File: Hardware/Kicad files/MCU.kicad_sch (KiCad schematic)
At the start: 1 part, among them U201 NUCLEO-H753ZI

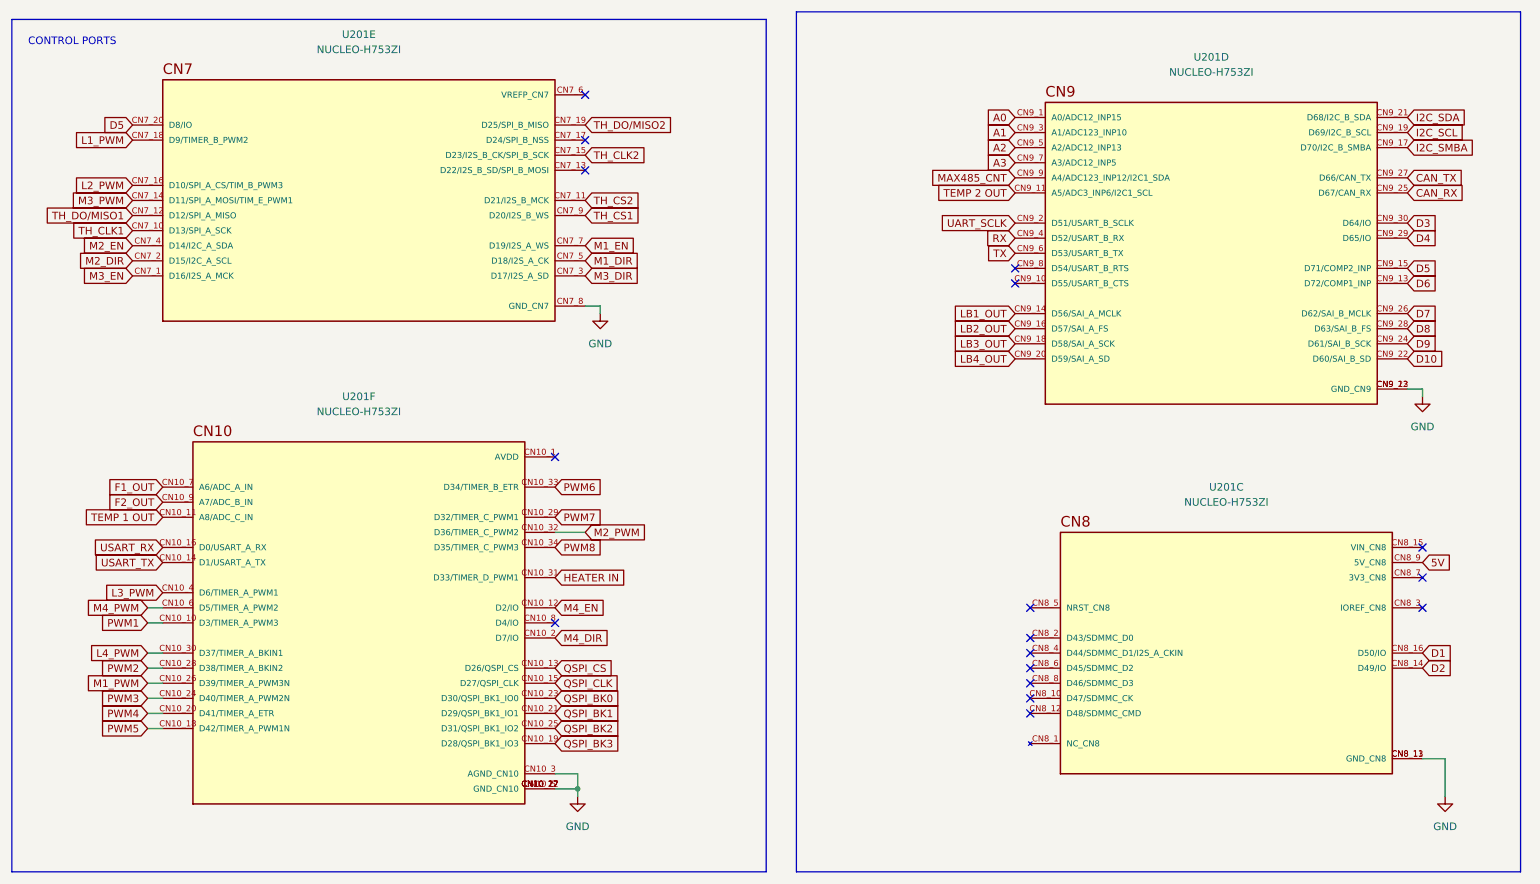
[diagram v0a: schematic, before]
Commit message: Add files via upload
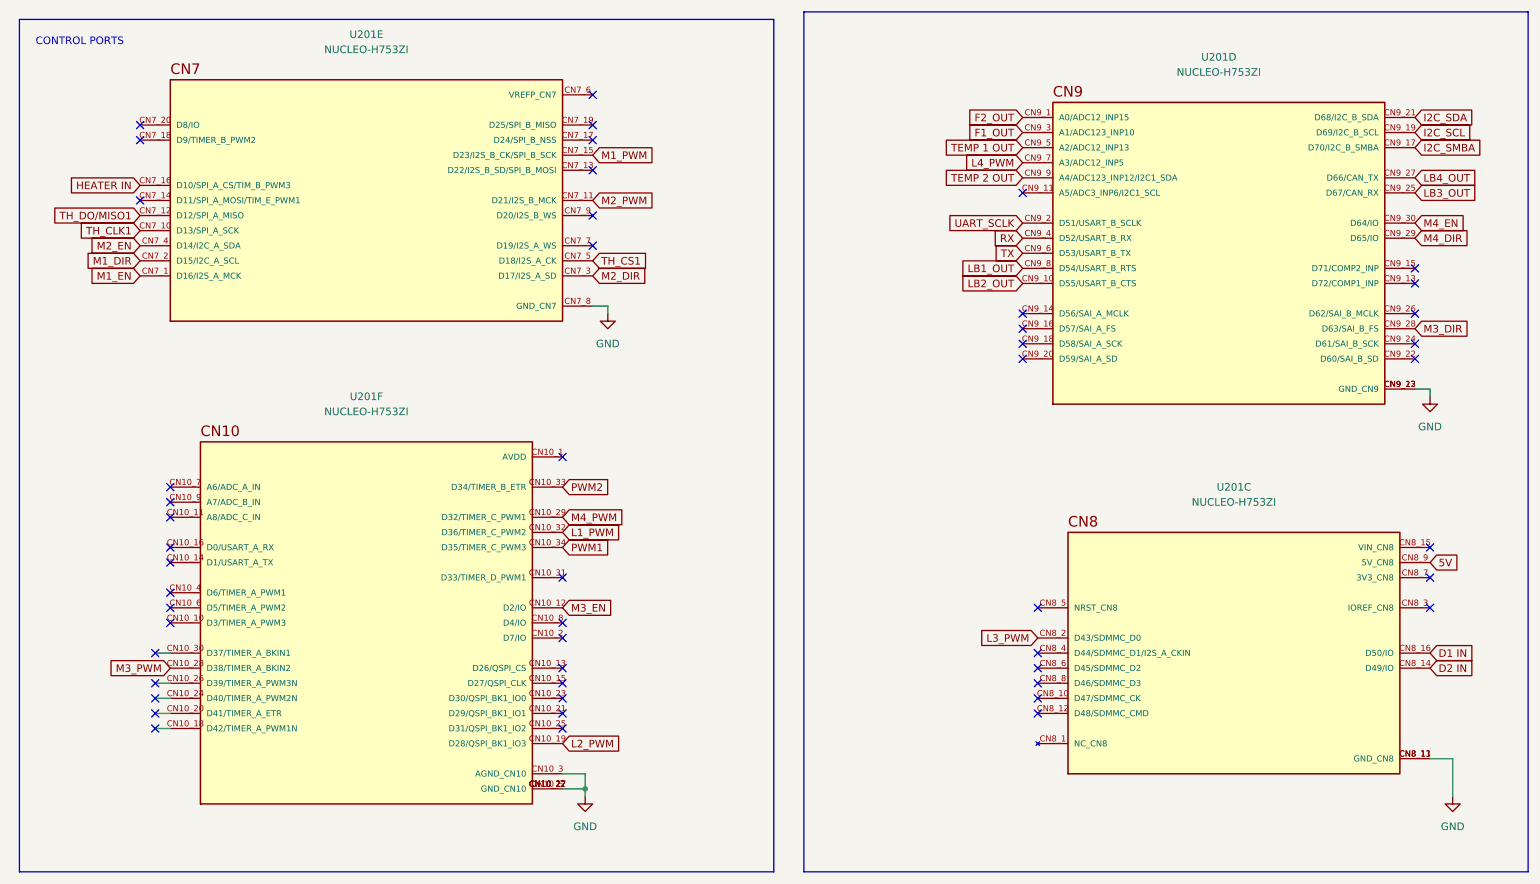
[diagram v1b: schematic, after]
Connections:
- net A0 is gone; now on net F2_OUT: U201.CN9_1 (A0/ADC12_INP15)
- net A1 is gone; now on net F1_OUT: U201.CN9_3 (A1/ADC123_INP10)
- net A2 is gone; now on net TEMP 1 OUT: U201.CN9_5 (A2/ADC12_INP13)
- net A3 is gone; now on net L4_PWM: U201.CN9_7 (A3/ADC12_INP5)
- net CAN_RX is gone; now on net LB3_OUT: U201.CN9_25 (D67/CAN_RX)
- net CAN_TX is gone; now on net LB4_OUT: U201.CN9_27 (D66/CAN_TX)
- net D3 is gone; now on net M4_EN: U201.CN9_30 (D64/IO)
- net D4 is gone; now on net M4_DIR: U201.CN9_29 (D65/IO)
- net D8 is gone; now on net M3_DIR: U201.CN9_28 (D63/SAI_B_FS)
- net MAX485_CNT is gone; now on net TEMP 2 OUT: U201.CN9_9 (A4/ADC123_INP12/I2C1_SDA)
- net PWM6 is gone; now on net PWM2: U201.CN10_33 (D34/TIMER_B_ETR)
- net PWM7 is gone; now on net M4_PWM: U201.CN10_29 (D32/TIMER_C_PWM1)
- net PWM8 is gone; now on net PWM1: U201.CN10_34 (D35/TIMER_C_PWM3)
- net QSPI_BK3 is gone; now on net L2_PWM: U201.CN10_19 (D28/QSPI_BK1_IO3)
- net TH_CLK2 is gone; now on net M1_PWM: U201.CN7_15 (D23/I2S_B_CK/SPI_B_SCK)
- net TH_CS2 is gone; now on net M2_PWM: U201.CN7_11 (D21/I2S_B_MCK)
- net F1_OUT: no longer U201.CN10_7 (A6/ADC_A_IN)
- net F2_OUT: no longer U201.CN10_9 (A7/ADC_B_IN)
- net HEATER IN: now also U201.CN7_16 (D10/SPI_A_CS/TIM_B_PWM3); no longer U201.CN10_31 (D33/TIMER_D_PWM1)
- net L1_PWM: now also U201.CN10_32 (D36/TIMER_C_PWM2); no longer U201.CN7_18 (D9/TIMER_B_PWM2)
- net L2_PWM: no longer U201.CN7_16 (D10/SPI_A_CS/TIM_B_PWM3)
- net L3_PWM: now also U201.CN8_2 (D43/SDMMC_D0); no longer U201.CN10_4 (D6/TIMER_A_PWM1)
- net L4_PWM: no longer U201.CN10_30 (D37/TIMER_A_BKIN1)
- net LB1_OUT: now also U201.CN9_8 (D54/USART_B_RTS); no longer U201.CN9_14 (D56/SAI_A_MCLK)
- net LB2_OUT: now also U201.CN9_10 (D55/USART_B_CTS); no longer U201.CN9_16 (D57/SAI_A_FS)
- net LB3_OUT: no longer U201.CN9_18 (D58/SAI_A_SCK)
- net LB4_OUT: no longer U201.CN9_20 (D59/SAI_A_SD)
- net M1_DIR: now also U201.CN7_2 (D15/I2C_A_SCL); no longer U201.CN7_5 (D18/I2S_A_CK)
- net M1_EN: now also U201.CN7_1 (D16/I2S_A_MCK); no longer U201.CN7_7 (D19/I2S_A_WS)
- net M1_PWM: no longer U201.CN10_26 (D39/TIMER_A_PWM3N)
- net M2_DIR: now also U201.CN7_3 (D17/I2S_A_SD); no longer U201.CN7_2 (D15/I2C_A_SCL)
- net M2_PWM: no longer U201.CN10_32 (D36/TIMER_C_PWM2)
- net M3_DIR: no longer U201.CN7_3 (D17/I2S_A_SD)
- net M3_EN: now also U201.CN10_12 (D2/IO); no longer U201.CN7_1 (D16/I2S_A_MCK)
- net M3_PWM: now also U201.CN10_28 (D38/TIMER_A_BKIN2); no longer U201.CN7_14 (D11/SPI_A_MOSI/TIM_E_PWM1)
- net M4_DIR: no longer U201.CN10_2 (D7/IO)
- net M4_EN: no longer U201.CN10_12 (D2/IO)
- net M4_PWM: no longer U201.CN10_6 (D5/TIMER_A_PWM2)
- net PWM1: no longer U201.CN10_10 (D3/TIMER_A_PWM3)
- net PWM2: no longer U201.CN10_28 (D38/TIMER_A_BKIN2)
- net TEMP 1 OUT: no longer U201.CN10_11 (A8/ADC_C_IN)
- net TEMP 2 OUT: no longer U201.CN9_11 (A5/ADC3_INP6/I2C1_SCL)
- net TH_CS1: now also U201.CN7_5 (D18/I2S_A_CK); no longer U201.CN7_9 (D20/I2S_B_WS)
- net D1 renamed D1 IN
- net D10: no longer names the net of U201.CN9_22 (D60/SAI_B_SD)
- net D2 renamed D2 IN
- net D5: no longer names the net of U201.CN9_15 (D71/COMP2_INP)
- net D5: no longer U201.CN7_20 (D8/IO)
- net D6: no longer names the net of U201.CN9_13 (D72/COMP1_INP)
- net D7: no longer names the net of U201.CN9_26 (D62/SAI_B_MCLK)
- net D9: no longer names the net of U201.CN9_24 (D61/SAI_B_SCK)
- net PWM3: no longer names the net of U201.CN10_24 (D40/TIMER_A_PWM2N)
- net PWM4: no longer names the net of U201.CN10_20 (D41/TIMER_A_ETR)
- net PWM5: no longer names the net of U201.CN10_18 (D42/TIMER_A_PWM1N)
- net QSPI_BK0: no longer names the net of U201.CN10_23 (D30/QSPI_BK1_IO0)
- net QSPI_BK1: no longer names the net of U201.CN10_21 (D29/QSPI_BK1_IO1)
- net QSPI_BK2: no longer names the net of U201.CN10_25 (D31/QSPI_BK1_IO2)
- net QSPI_CLK: no longer names the net of U201.CN10_15 (D27/QSPI_CLK)
- net QSPI_CS: no longer names the net of U201.CN10_13 (D26/QSPI_CS)
- net TH_DO/MISO2: no longer names the net of U201.CN7_19 (D25/SPI_B_MISO)
- net USART_RX: no longer names the net of U201.CN10_16 (D0/USART_A_RX)
- net USART_TX: no longer names the net of U201.CN10_14 (D1/USART_A_TX)
- no-connect marks 17 -> 50

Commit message: Add files via upload
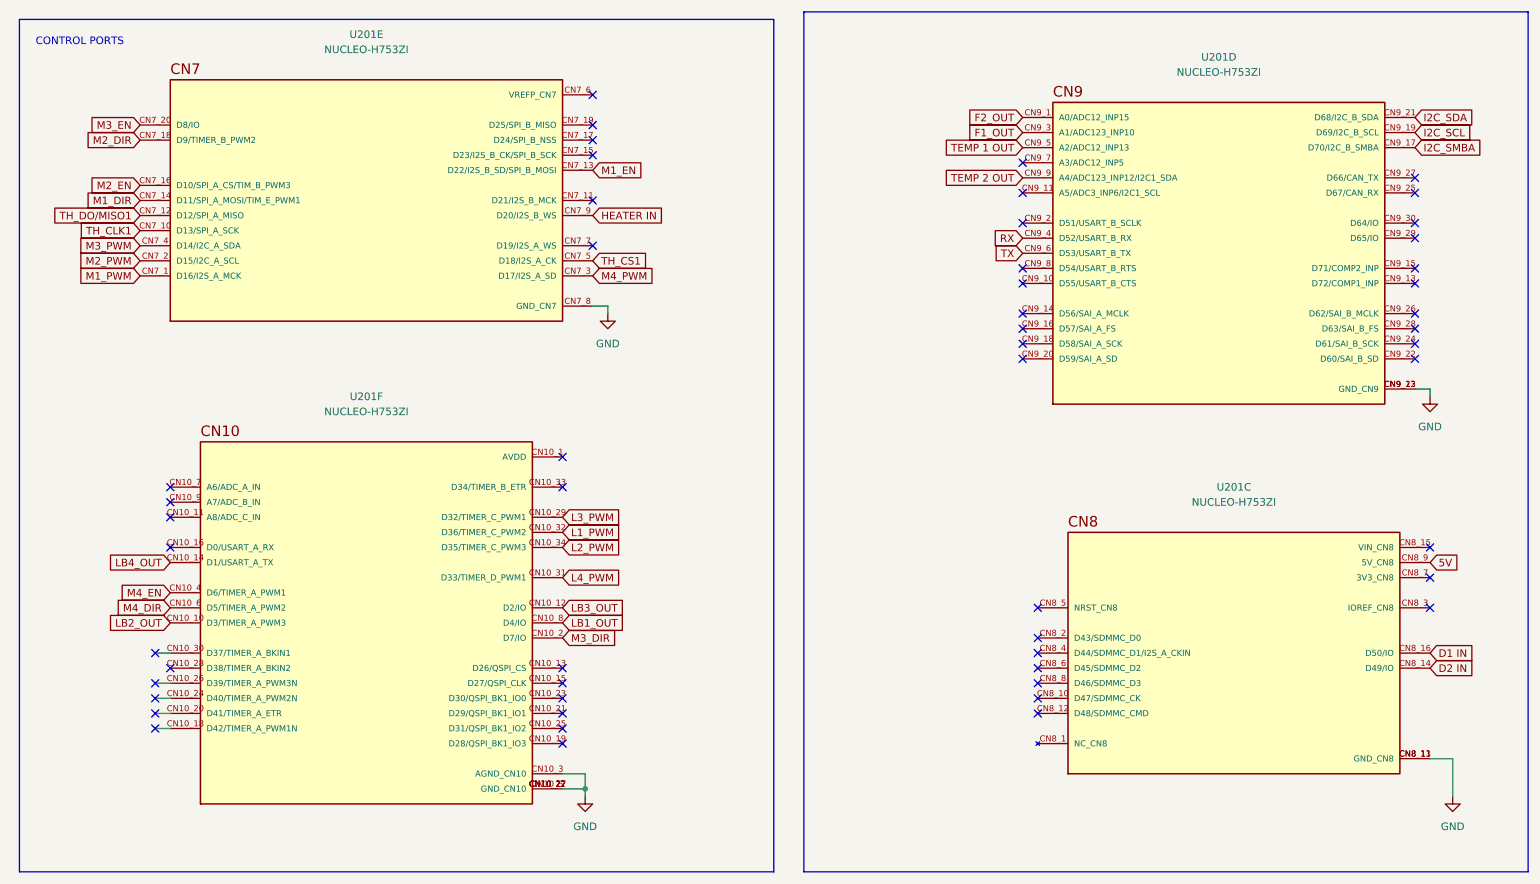
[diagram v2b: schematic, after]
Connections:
- net PWM1 is gone; now on net L2_PWM: U201.CN10_34 (D35/TIMER_C_PWM3)
- net HEATER IN: now also U201.CN7_9 (D20/I2S_B_WS); no longer U201.CN7_16 (D10/SPI_A_CS/TIM_B_PWM3)
- net L2_PWM: no longer U201.CN10_19 (D28/QSPI_BK1_IO3)
- net L3_PWM: now also U201.CN10_29 (D32/TIMER_C_PWM1); no longer U201.CN8_2 (D43/SDMMC_D0)
- net L4_PWM: now also U201.CN10_31 (D33/TIMER_D_PWM1); no longer U201.CN9_7 (A3/ADC12_INP5)
- net LB1_OUT: now also U201.CN10_8 (D4/IO); no longer U201.CN9_8 (D54/USART_B_RTS)
- net LB2_OUT: now also U201.CN10_10 (D3/TIMER_A_PWM3); no longer U201.CN9_10 (D55/USART_B_CTS)
- net LB3_OUT: now also U201.CN10_12 (D2/IO); no longer U201.CN9_25 (D67/CAN_RX)
- net LB4_OUT: now also U201.CN10_14 (D1/USART_A_TX); no longer U201.CN9_27 (D66/CAN_TX)
- net M1_DIR: now also U201.CN7_14 (D11/SPI_A_MOSI/TIM_E_PWM1); no longer U201.CN7_2 (D15/I2C_A_SCL)
- net M1_EN: now also U201.CN7_13 (D22/I2S_B_SD/SPI_B_MOSI); no longer U201.CN7_1 (D16/I2S_A_MCK)
- net M1_PWM: now also U201.CN7_1 (D16/I2S_A_MCK); no longer U201.CN7_15 (D23/I2S_B_CK/SPI_B_SCK)
- net M2_DIR: now also U201.CN7_18 (D9/TIMER_B_PWM2); no longer U201.CN7_3 (D17/I2S_A_SD)
- net M2_EN: now also U201.CN7_16 (D10/SPI_A_CS/TIM_B_PWM3); no longer U201.CN7_4 (D14/I2C_A_SDA)
- net M2_PWM: now also U201.CN7_2 (D15/I2C_A_SCL); no longer U201.CN7_11 (D21/I2S_B_MCK)
- net M3_DIR: now also U201.CN10_2 (D7/IO); no longer U201.CN9_28 (D63/SAI_B_FS)
- net M3_EN: now also U201.CN7_20 (D8/IO); no longer U201.CN10_12 (D2/IO)
- net M3_PWM: now also U201.CN7_4 (D14/I2C_A_SDA); no longer U201.CN10_28 (D38/TIMER_A_BKIN2)
- net M4_DIR: now also U201.CN10_6 (D5/TIMER_A_PWM2); no longer U201.CN9_29 (D65/IO)
- net M4_EN: now also U201.CN10_4 (D6/TIMER_A_PWM1); no longer U201.CN9_30 (D64/IO)
- net M4_PWM: now also U201.CN7_3 (D17/I2S_A_SD); no longer U201.CN10_29 (D32/TIMER_C_PWM1)
- net PWM2: no longer names the net of U201.CN10_33 (D34/TIMER_B_ETR)
- net UART_SCLK: no longer names the net of U201.CN9_2 (D51/USART_B_SCLK)
- no-connect marks 50 -> 53

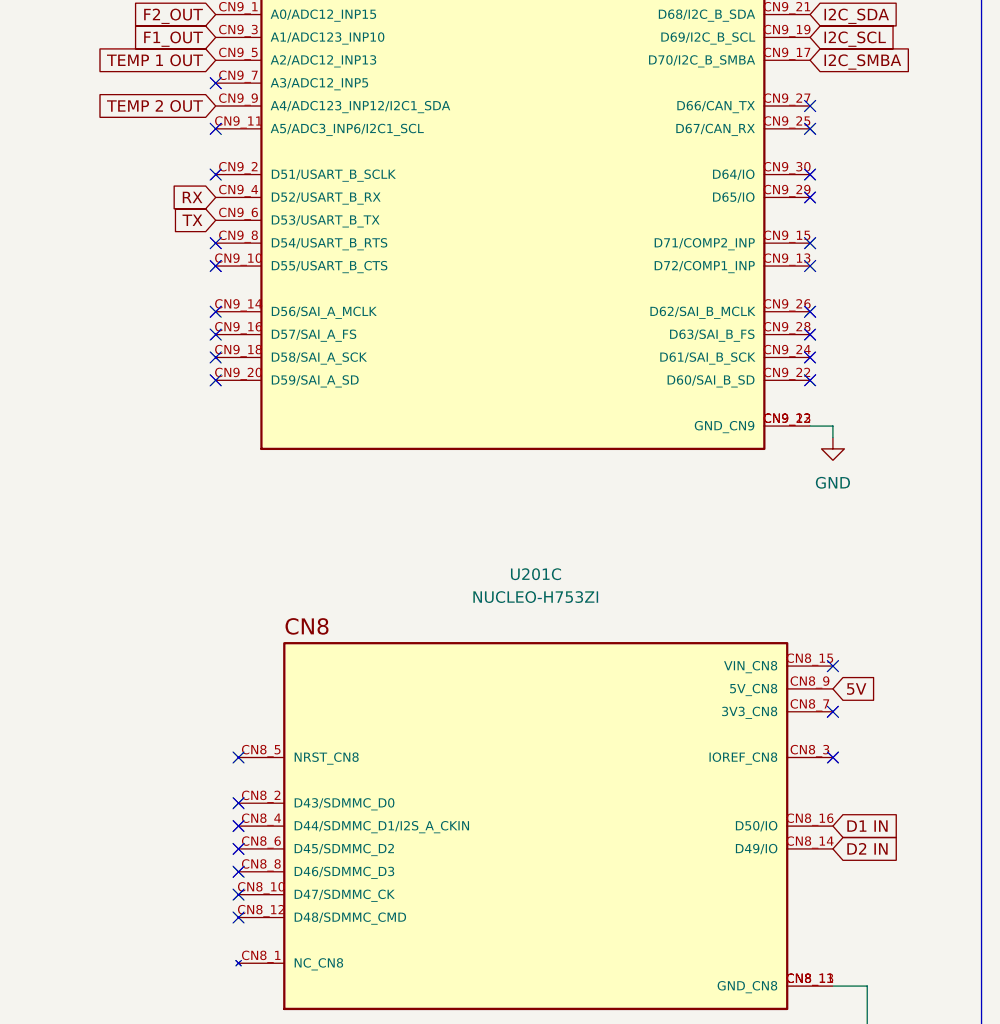
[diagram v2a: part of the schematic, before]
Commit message: includes the modifications made
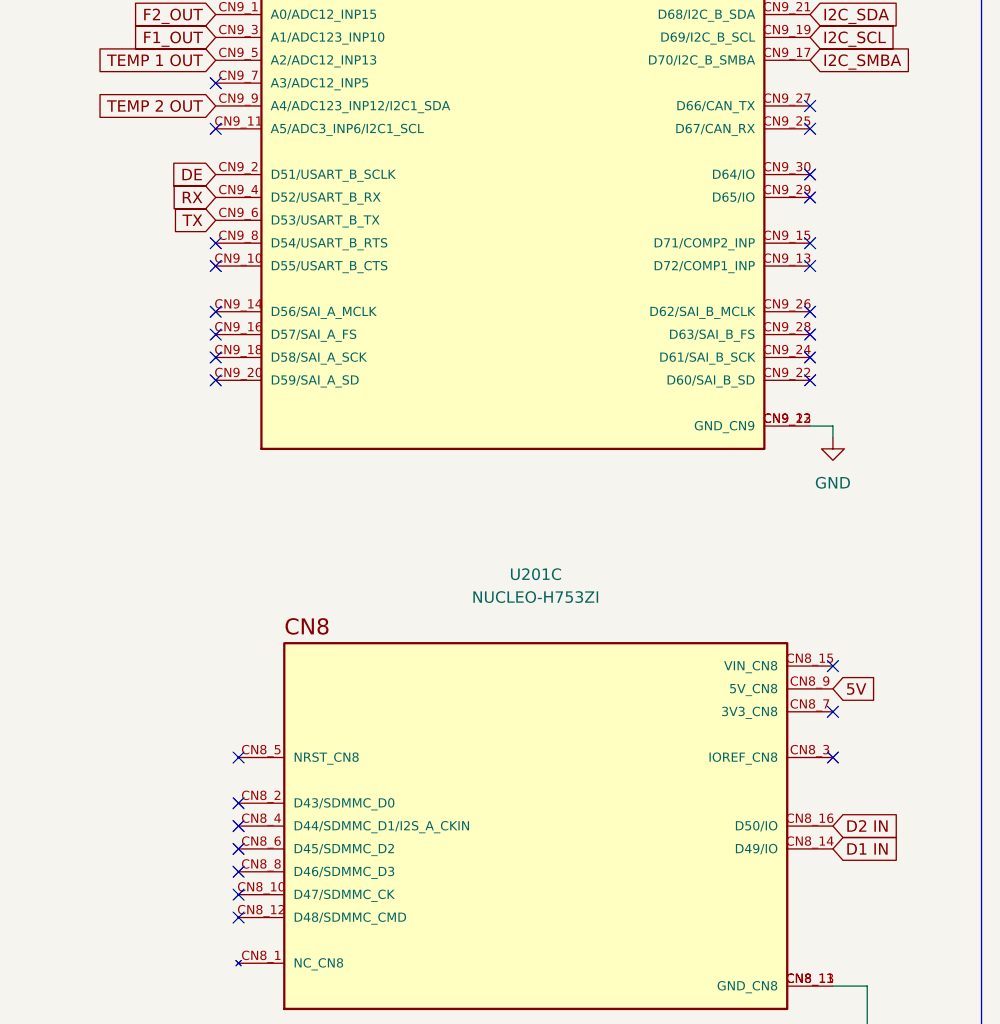
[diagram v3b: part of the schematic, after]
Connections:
- net D1 IN: now also U201.CN8_14 (D49/IO); no longer U201.CN8_16 (D50/IO)
- net D2 IN: now also U201.CN8_16 (D50/IO); no longer U201.CN8_14 (D49/IO)
- net DE: now reaches U201.CN9_2 (D51/USART_B_SCLK)
- no-connect marks 53 -> 52
